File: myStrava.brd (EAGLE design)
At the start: 64.8 x 45.4 mm, 43 parts, among them Y1 16MHz

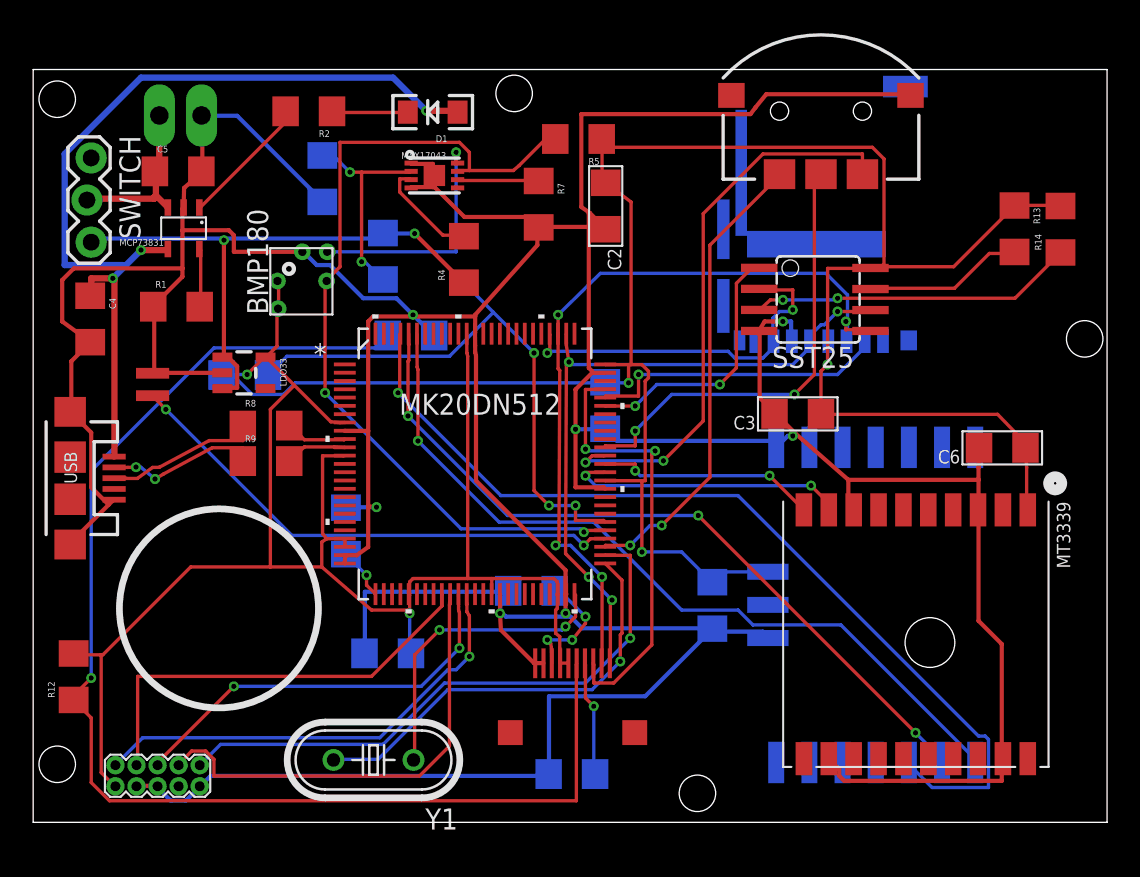
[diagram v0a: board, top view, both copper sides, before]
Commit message: Avant autoroutage
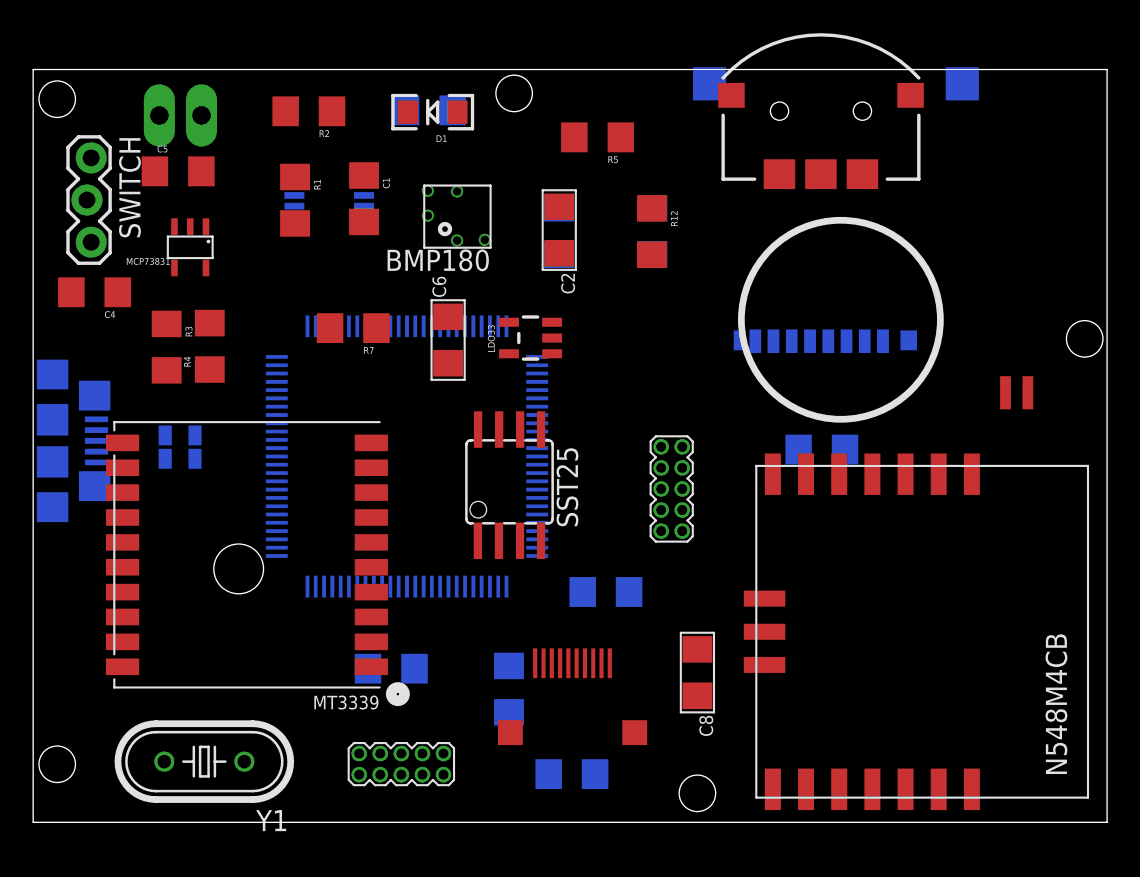
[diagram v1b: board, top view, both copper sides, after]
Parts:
- removed MAX17043: MAX1704X, SparkFun-PowerIC:TDFN-8
- removed R13, R14: 10k, SparkFun-Resistors:1206
- added JTAG1: 2X5_0.05"_CORTEX_DEBUGTH_NOKEY_UNSHROUDED, con-cortex:2X5_0.05"_TH_NS
- added U$1: STC3100, STC3100:STC3100
- C1: value 1uF -> 220nF
- C4, C5: value 4.7uF -> 10uF
- R3: value 1k -> 200k/0.1%
- R4: value 180 -> 0.02
- R7: value 4.7k -> 1kOhms
- R8, R9: device SparkFun-Resistors:1206 -> SparkFun-Resistors:0805
- moved SPK 52.1 mm to (60.3, 26.9), turned to 180 degrees
- moved R12 44.0 mm to (37.3, 35.6), turned to 270 degrees
- moved MT3339 40.6 mm to (12.9, 16.1), turned to 180 degrees
- moved C6 34.0 mm to (25.0, 29.1), turned to 90 degrees
- moved N550 21.6 mm to (63.6, 1.49), flipped to the top, turned to 90 degrees
- moved R6 19.5 mm to (23.9, 42.9), turned to 0 degrees
- moved SST25 17.4 mm to (31.3, 15.4), turned to 90 degrees
- moved LDO33 17.4 mm to (30.0, 29.2), turned to 90 degrees
- moved R4 16.2 mm to (10.7, 28.7)
- moved JTAG 14.7 mm to (22.2, 3.51)
- moved R3 14.1 mm to (8.05, 28.6), flipped to the top
- moved C10 13.7 mm to (28.7, 8.03), turned to 270 degrees
- moved C7 13.7 mm to (34.5, 13.9)
- moved R7 13.4 mm to (19.3, 29.8), turned to 180 degrees
- moved C11 10.9 mm to (31.7, 35.6), turned to 270 degrees
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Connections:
- removed net N$29: MK20DN512.64, NAV.2
- removed net N$30: MK20DN512.65, NAV.T
- removed net N$31: MK20DN512.53, NAV.1
- removed net N$33: R14.1, SST25.WP
- removed net N$34: R13.2, SST25.HOLD
- new net N$10: N550.NONE1, NAV.2
- new net N$11: N550.SUSPEND, NAV.T
- new net N$12: N550.SLEEP, NAV.1
- new net N$13: N550.NONE2, NAV.C
- new net N$15: MK20DN512.69, SST25.WP
- new net N$24: MK20DN512.68, SST25.HOLD
- new net N$5: C1.1, R7.1, U$1.VIN
- new net N$6: BATT.2, R4.2, U$1.CG
- new net N$9: N550.PORTSEL, SPK.P$2
- new net VCC: JTAG1.1
- net GND: now also C1.2, JTAG1.3, JTAG1.5, JTAG1.9, R3.2, R4.1, U$1.GND; no longer BATT.2, C1.1, MAX17043.1, MAX17043.4, MAX17043.EP, NAV.C, R7.2, SPK.P$2
- net MK_SCL: now also U$1.SCL; no longer MAX17043.7
- net MK_SDA: now also U$1.SDA; no longer MAX17043.8
- net N$3: now also JTAG1.2, N550.RST; no longer MK20DN512.54, SPK.P$1
- net N$4: now also R3.1, U$1.ROSC; no longer C1.2, MAX17043.2, R3.2
- net N$7: now also JTAG1.4, N550.P$12; no longer MAX17043.3, R4.2
- net N$8: now also N550.SCLK, SPK.P$1; no longer MAX17043.6, R7.1
- net VCC-ISO: now also R7.2, U$1.VCC; no longer R3.1, R4.1
- net VDD: no longer R13.1, R14.2
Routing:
- net GND: track 341.7 -> 0.00 mm, vias 7 -> 0
- net VDD: track 236.5 -> 0.00 mm, vias 5 -> 0
- net N$27: track 78.9 -> 0.00 mm, vias 1 -> 0
- net N$21: track 56.3 -> 0.00 mm, vias 1 -> 0
- net N$18: track 54.0 -> 0.00 mm, vias 3 -> 0
- net MK_SDA: track 52.1 -> 0.00 mm, vias 4 -> 0
- net MK_SCL: track 51.8 -> 0.00 mm, vias 2 -> 0
- net MK_RX3: track 48.2 -> 0.00 mm, vias 1 -> 0
- net MK_DO: track 46.8 -> 0.00 mm, vias 4 -> 0
- net MK_TX3: track 45.9 -> 0.00 mm, vias 3 -> 0
- net MK_SCLK: track 41.2 -> 0.00 mm, vias 4 -> 0
- net N$35: track 35.6 -> 0.00 mm, vias 1 -> 0
- net VCC-ISO: track 34.4 -> 0.00 mm, vias 2 -> 0
- net N$29: track 34.3 -> 0.00 mm, vias 2 -> 0
- net N$3: track 31.2 -> 0.00 mm, vias 2 -> 0
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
